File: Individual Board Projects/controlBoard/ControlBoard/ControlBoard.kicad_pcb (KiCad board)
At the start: 2 copper layers, 120 x 116.2 mm, 11 parts, among them J1 USBCPD, J3 5x2.54mm+2xBus, J4 MJ1-2503A, U1 LMC6484IN_NOPB, U2 01000020Z, U3 ESP32-C6-DEVKITC-1-N8

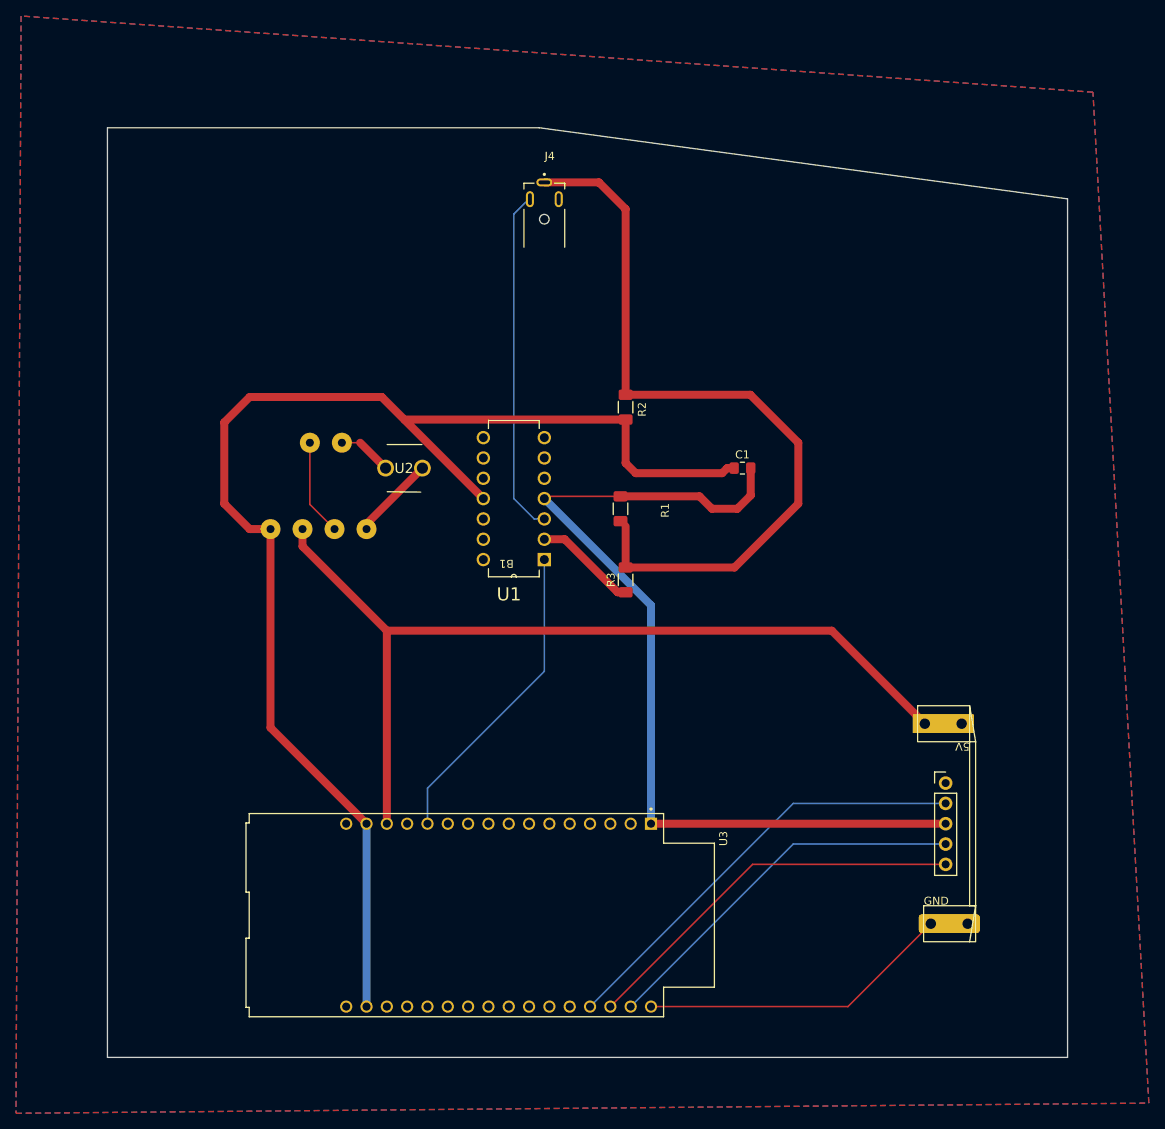
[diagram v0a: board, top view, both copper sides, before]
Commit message: Updated ControlBoard design files
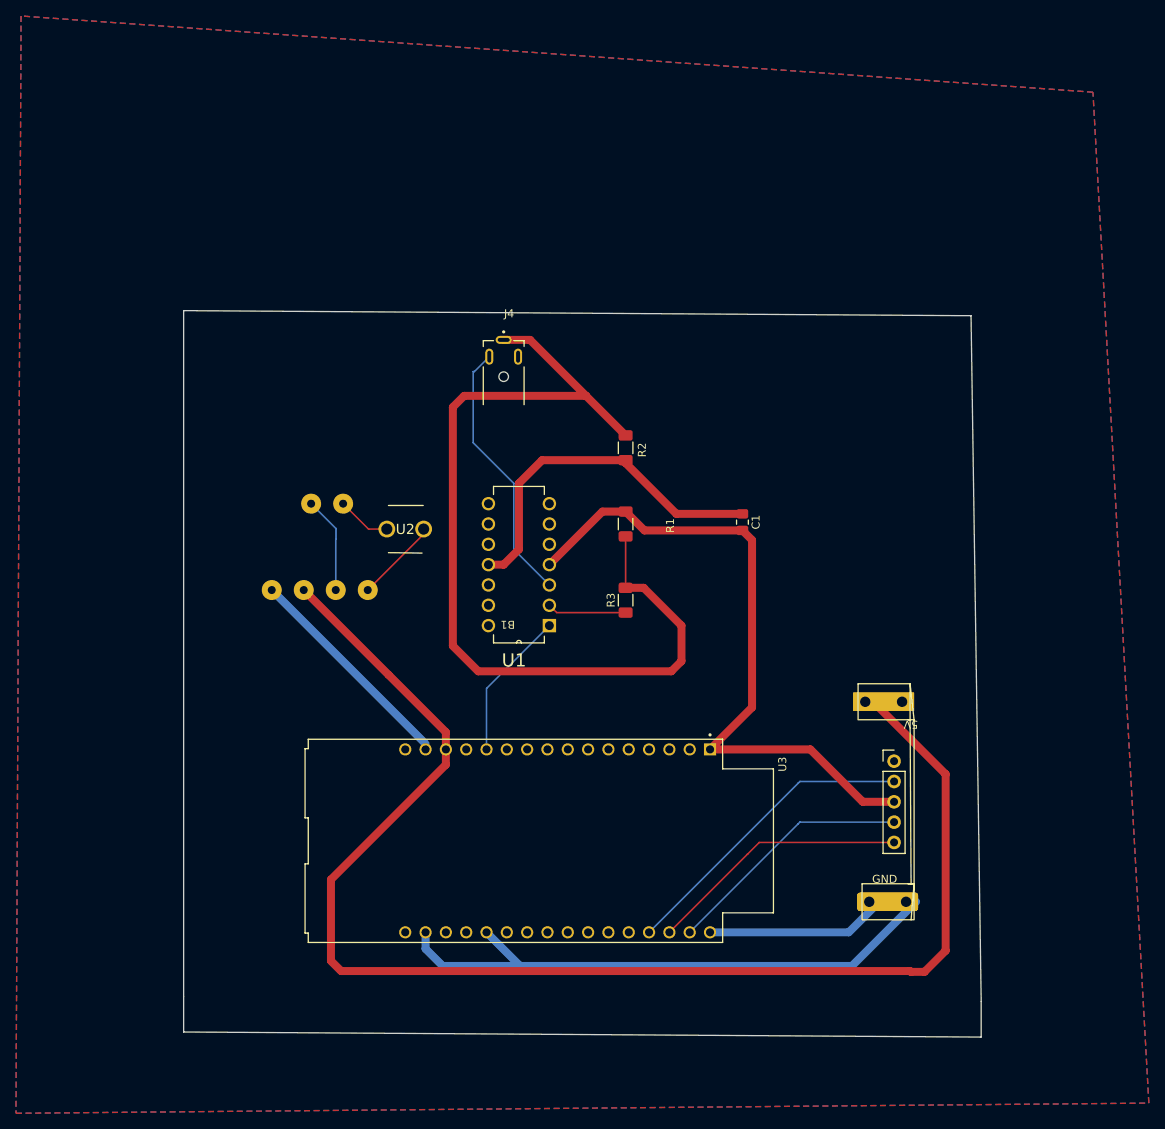
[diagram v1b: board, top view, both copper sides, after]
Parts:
- moved J4 20.3 mm to (138.4, 64.1)
- moved U3 11.9 mm to (139.9, 122.2)
- moved U1 8.28 mm to (136.5, 80.0)
- moved B1 7.62 mm to (117.4, 90.8)
- moved J1 7.62 mm to (114.4, 80.0)
- moved U2 7.62 mm to (123.8, 83.2)
- moved J3 7.00 mm to (187.2, 117.3)
- moved C1 6.75 mm to (168.3, 82.3), turned to -90 degrees
- moved R2 5.08 mm to (153.7, 73.0)
- moved R3 2.54 mm to (153.7, 92.1)
- moved R1 2.01 mm to (153.7, 82.5)
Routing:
- net +5V: track 113.3 -> 173.0 mm
- net GND: track 207.6 -> 169.1 mm
- net +3.3V: track 113.7 -> 83.6 mm
- net /To ESP32 ADC: track 39.1 -> 18.7 mm
- net +1.65V: track 97.4 -> 117.5 mm
- net /ESP32_UART_RX: track 49.3 -> 32.7 mm
- net /nShoutRecive: track 55.0 -> 38.4 mm
- net /ESP32_UART_TX: track 47.8 -> 31.2 mm
- net Net-(U1-POS1): track 43.2 -> 33.4 mm
- net Net-(U1-NEG1): track 12.9 -> 9.90 mm
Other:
- board size 120 x 116.2 mm -> 99.7 x 90.8 mm

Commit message: Updated ControlBoard design files
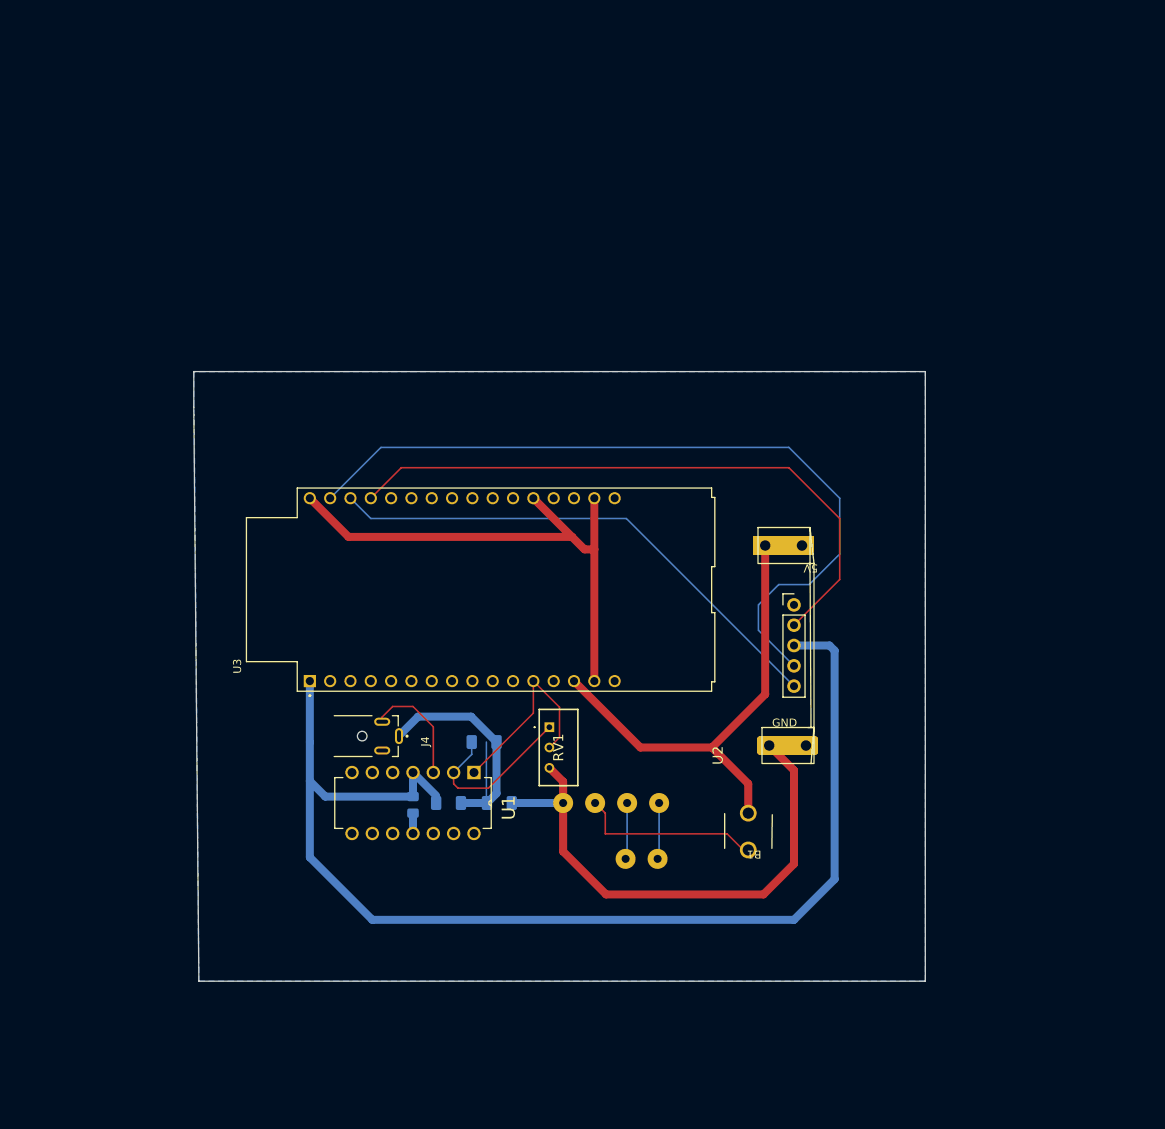
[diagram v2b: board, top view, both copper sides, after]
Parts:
- added RV1: 1-400k, BUCK_and_USBC:Potentiometer, F.Cu at (144.1, 108.0)
- C1, R1, R2, R3: moved to B.Cu
- moved U2 60.4 mm to (169.0, 123.3), turned to 90 degrees
- moved J1 59.3 mm to (153.7, 124.4)
- moved C1 54.3 mm to (127.1, 117.7), turned to 90 degrees
- moved J4 48.3 mm to (120.7, 109.1), turned to -90 degrees
- moved R2 47.1 mm to (137.9, 117.4), turned to 0 degrees
- moved B1 45.1 mm to (153.9, 117.4)
- moved U1 44.6 mm to (119.5, 121.2), turned to -90 degrees
- moved R1 41.3 mm to (131.5, 117.4), turned to 0 degrees
- moved U3 31.4 mm to (138.5, 90.8), turned to 90 degrees
- moved R3 25.0 mm to (136.0, 109.8), turned to 0 degrees
- moved J3 23.2 mm to (174.7, 97.7)
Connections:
- B1 pad 3: +5V -> Net-(B1-+Vout)
- J1 pad 1: Net-(J1-Pin_1) -> /USBC+
- U2 pad 1: Net-(J1-Pin_1) -> Net-(B1-+Vout)
- U2 pad 2: /USBC+ -> +5V
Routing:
- net +5V: track 173.0 -> 58.8 mm
- net +1.65V: track 117.5 -> 33.6 mm
- net /ESP32_UART_TX: track 31.2 -> 98.2 mm
- net +3.3V: track 83.6 -> 148.6 mm
- net /nShoutRecive: track 38.4 -> 78.5 mm
- net /ESP32_UART_RX: track 32.7 -> 65.2 mm
- net GND: track 169.1 -> 136.8 mm
- net Net-(B1-+Vout): track 0.00 -> 22.3 mm
- net Net-(U1-POS1): track 33.4 -> 14.3 mm
- net Net-(U1-NEG1): track 9.90 -> 21.5 mm
- net Net-(J1-Pin_1): track 6.78 -> 0.00 mm
- net /To ESP32 ADC: track 18.7 -> 24.7 mm
- net /USBC-: track 12.1 -> 7.06 mm
- net /USBC+: track 10.5 -> 7.06 mm
- removed copper zone on F.Cu, net +5V
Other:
- board size 99.7 x 90.8 mm -> 91.4 x 76.2 mm

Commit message: Controll Finished - READY TO FAB
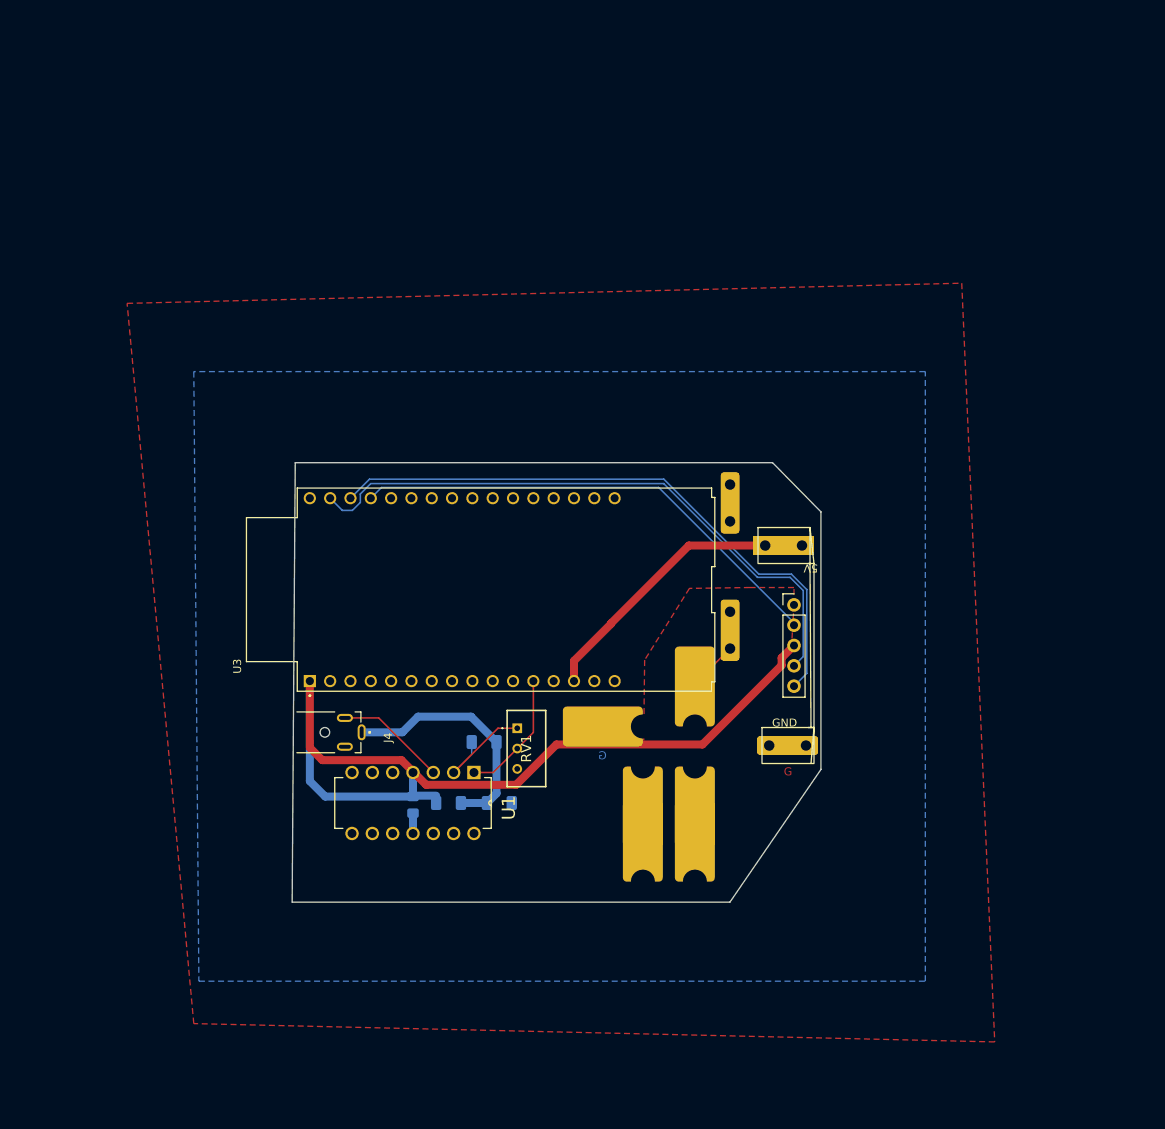
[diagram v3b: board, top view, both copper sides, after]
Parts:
- moved U2 36.3 mm to (166.9, 87.0)
- moved J1 8.97 mm to (159.1, 117.3), turned to 90 degrees
- moved B1 8.78 mm to (159.1, 110.4), turned to 90 degrees
- moved J4 4.69 mm to (116.1, 108.6)
- moved RV1 4.02 mm to (140.1, 108.1)
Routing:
- net GND: track 136.8 -> 2.54 mm
- net +3.3V: track 148.6 -> 114.4 mm
- net +5V: track 58.8 -> 32.4 mm
- net /ESP32_UART_TX: track 98.2 -> 77.2 mm
- net /nShoutRecive: track 78.5 -> 60.8 mm
- net /ESP32_UART_RX: track 65.2 -> 76.5 mm
- net Net-(B1-+Vout): track 22.3 -> 11.6 mm
- net /To ESP32 ADC: track 24.7 -> 15.9 mm
- net /USBC-: track 7.06 -> 0.00 mm
- net /USBC+: track 7.06 -> 0.00 mm
- net Net-(U1-NEG1): track 21.5 -> 15.0 mm
- net +1.65V: track 33.6 -> 30.5 mm
- added copper zone on F.Cu, net +5V
- added copper zone on F.Cu, net Net-(B1-+Vout)
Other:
- board size 91.4 x 76.2 mm -> 66.1 x 54.9 mm
- board text added: "G"
